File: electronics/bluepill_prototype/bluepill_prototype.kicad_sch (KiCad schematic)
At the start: 16 parts, among them K1 Fujitsu_FTR-LYCA005x, M1 Motor_DC, SW1 SW_SPST, U1 Open_drain_hall_sensor, U2 YAAJ_BluePill_Part_Like, U3 MCP40D17

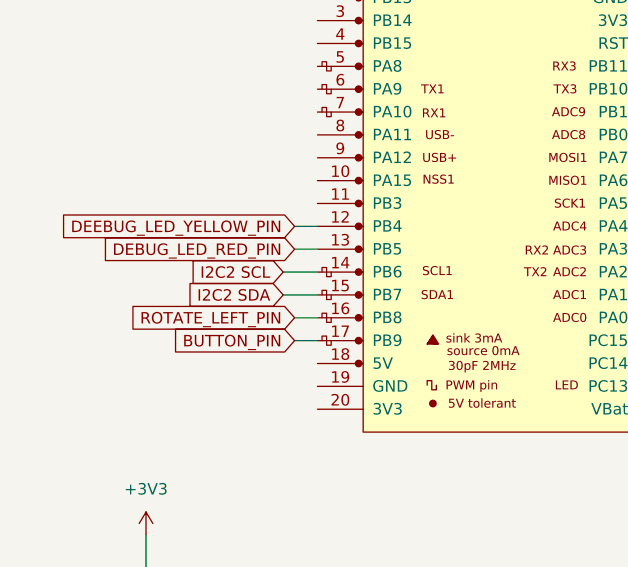
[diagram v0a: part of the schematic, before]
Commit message: fixed code
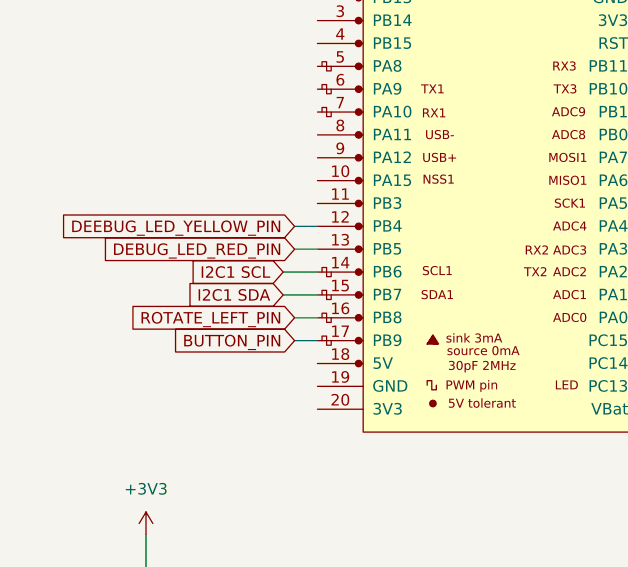
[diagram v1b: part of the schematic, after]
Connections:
- net I2C SCL: no longer U2.14 (PB6)
- net I2C SDA: no longer U2.15 (PB7)
- new net I2C1 SCL: U2.14 (PB6)
- new net I2C1 SDA: U2.15 (PB7)
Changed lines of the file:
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@@
 		)
 	)
-	(global_label "I2C2 SDA"
+	(global_label "I2C1 SDA"
 		(shape input)
 		(at 40.64 68.58 180)
@@
 		)
 	)
-	(global_label "I2C2 SCL"
+	(global_label "I2C1 SCL"
 		(shape input)
 		(at 40.64 66.04 180)
